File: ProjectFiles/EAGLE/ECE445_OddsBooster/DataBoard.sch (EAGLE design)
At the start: 51 parts, among them U2 74LV164D-SHIFT_REGISTER, U3 74LV164D-SHIFT_REGISTER, U4 74LV164D-SHIFT_REGISTER, X1 FH12-40S-0.5SH

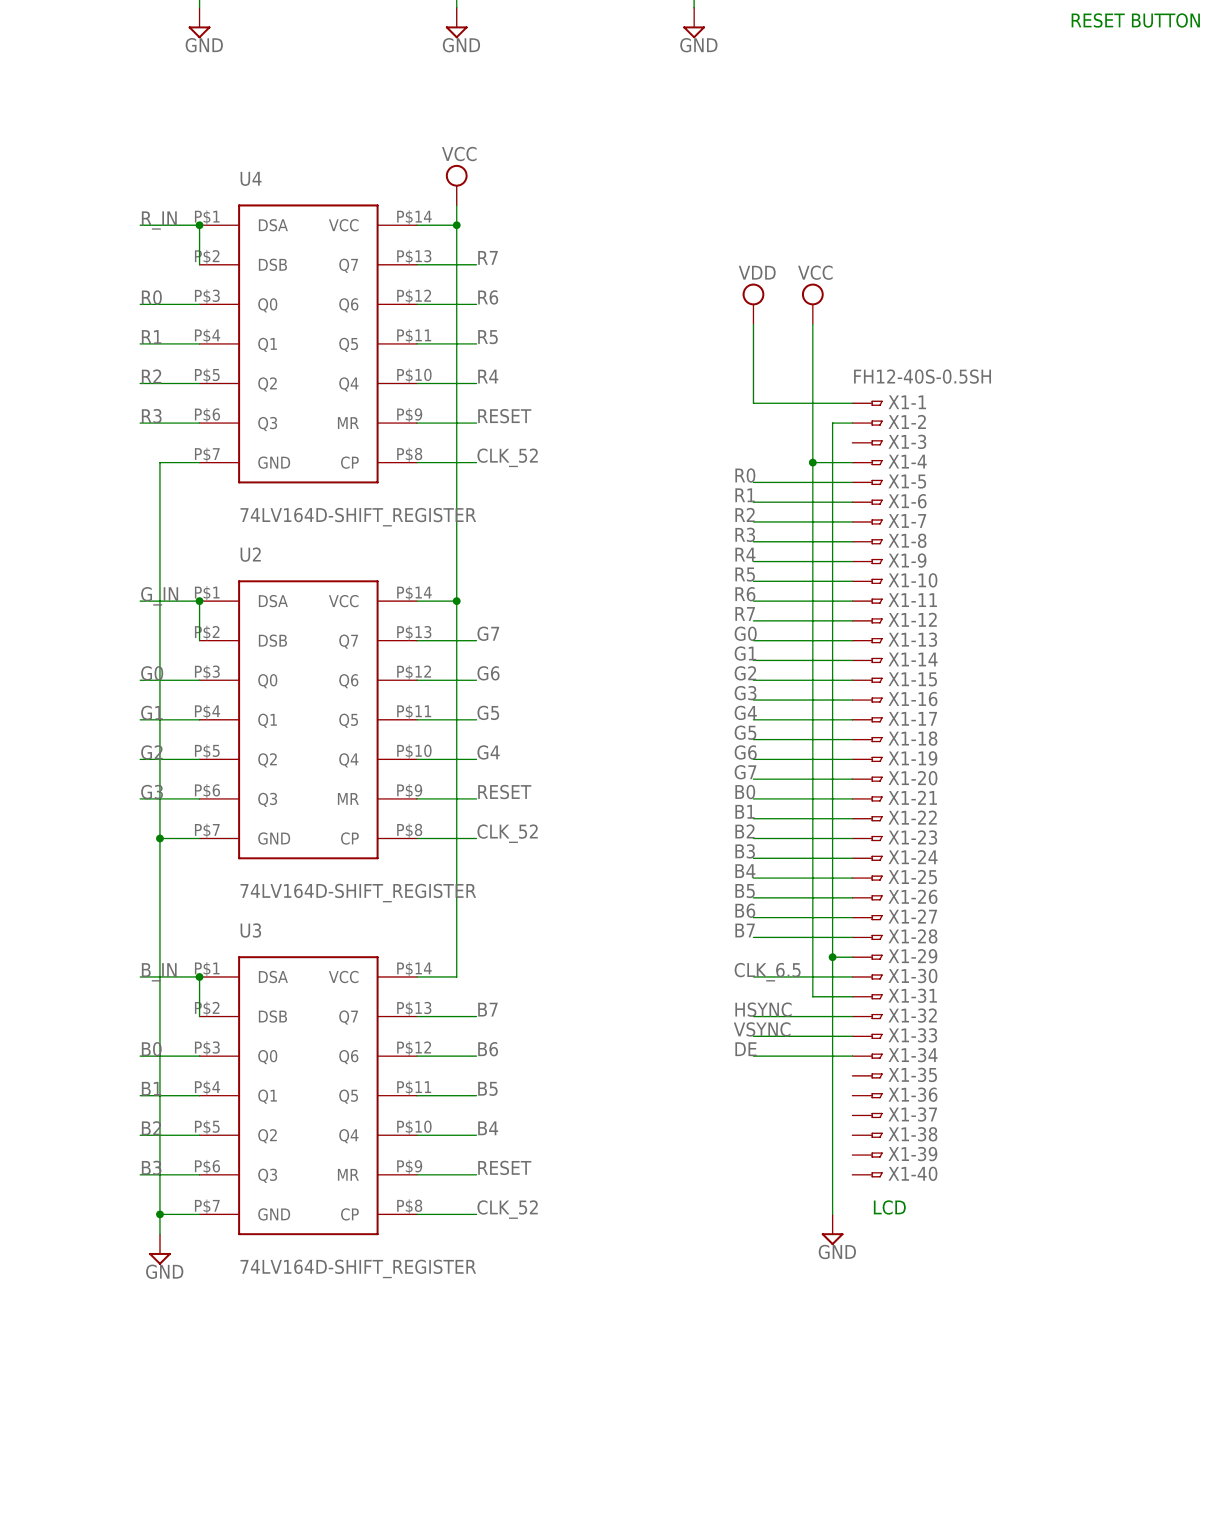
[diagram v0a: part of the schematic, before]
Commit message: layout minor changes
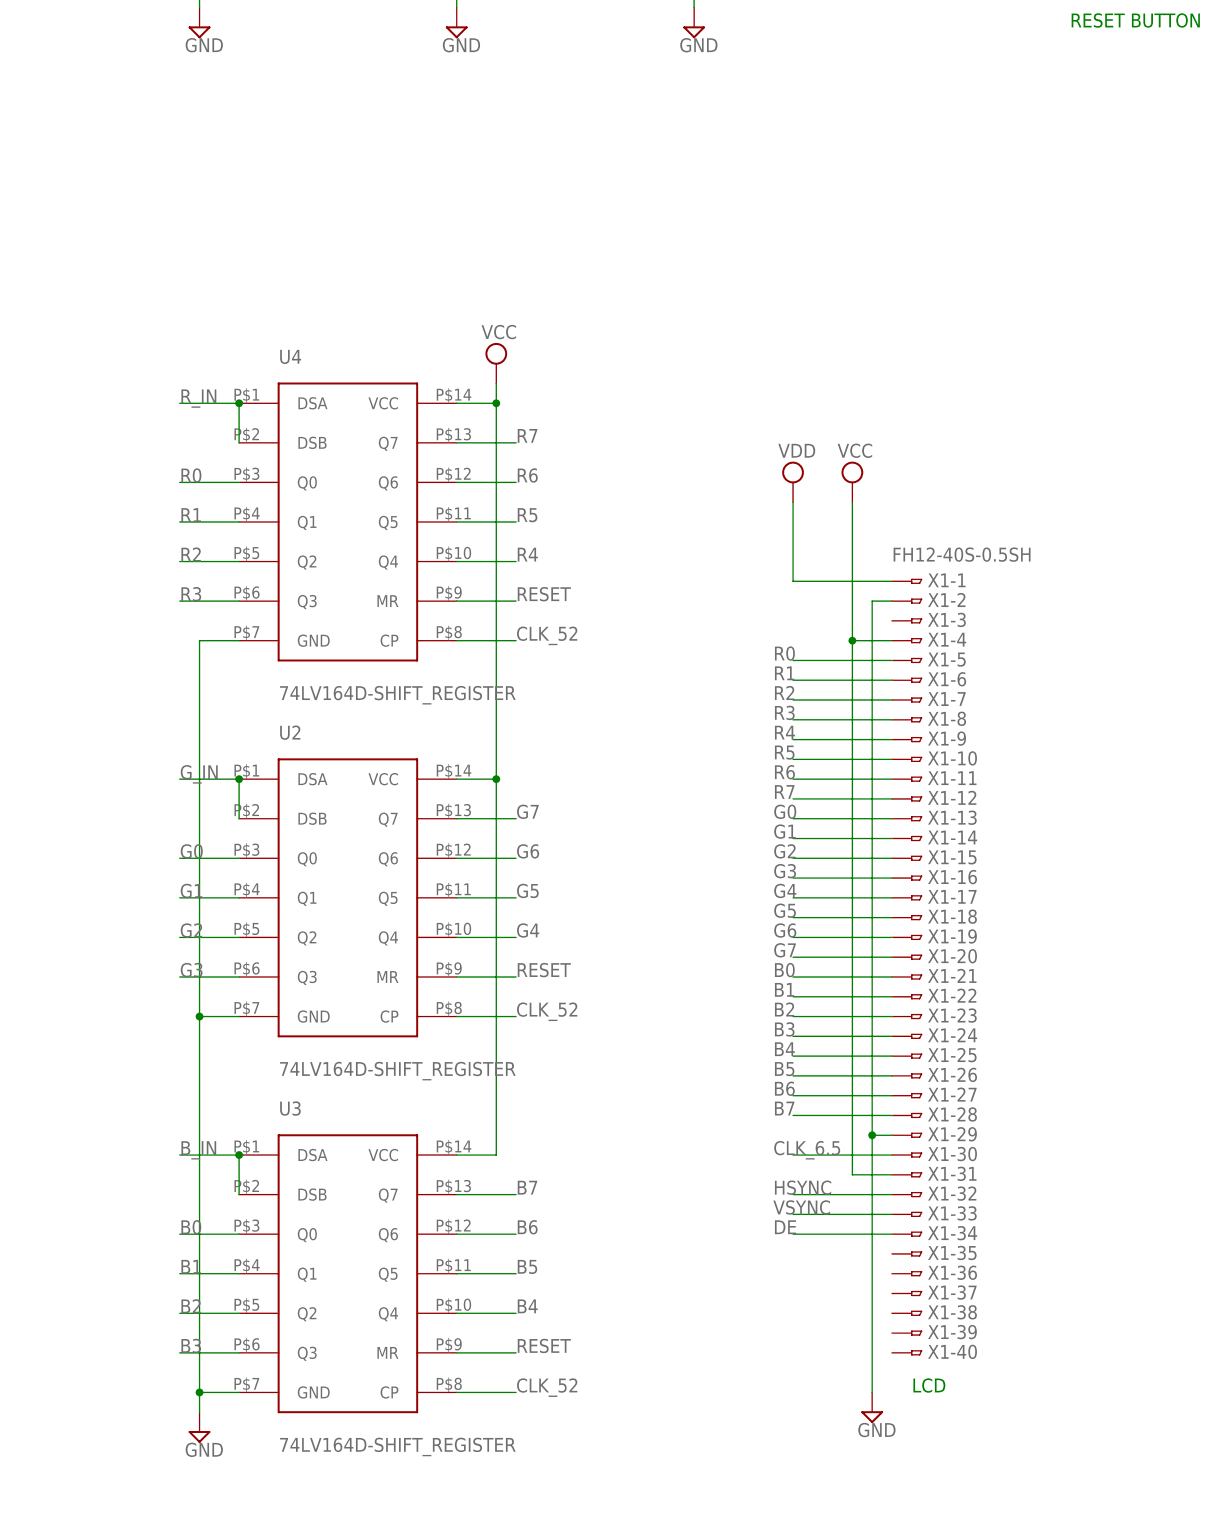
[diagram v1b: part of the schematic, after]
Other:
- moved on the sheet: U2, U3, U4, X1-1, X1-10, X1-11, X1-12, X1-13, X1-14, X1-15, X1-16, X1-17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
